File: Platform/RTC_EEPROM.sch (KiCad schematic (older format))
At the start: 21 parts, among them U4 DS3231M, U5 AT24CS32-SSHM, U6 MCP7940N-xMS, Y1 32KHz crystal

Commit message: updated.
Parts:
- BAT1: symbol Platform-rescue:BS-7-dk_Battery-Holders-Clips-Contacts -> Platform-rescue:BS-7-dk_Battery-Holders-Clips-Contacts-Platform-rescue
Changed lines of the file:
@@
 $EndComp
 $Comp
-L Platform-rescue:BS-7-dk_Battery-Holders-Clips-Contacts BAT1
+L Platform-rescue:BS-7-dk_Battery-Holders-Clips-Contacts-Platform-rescue BAT1
 U 1 1 5FB40A5C
 P 7500 1650

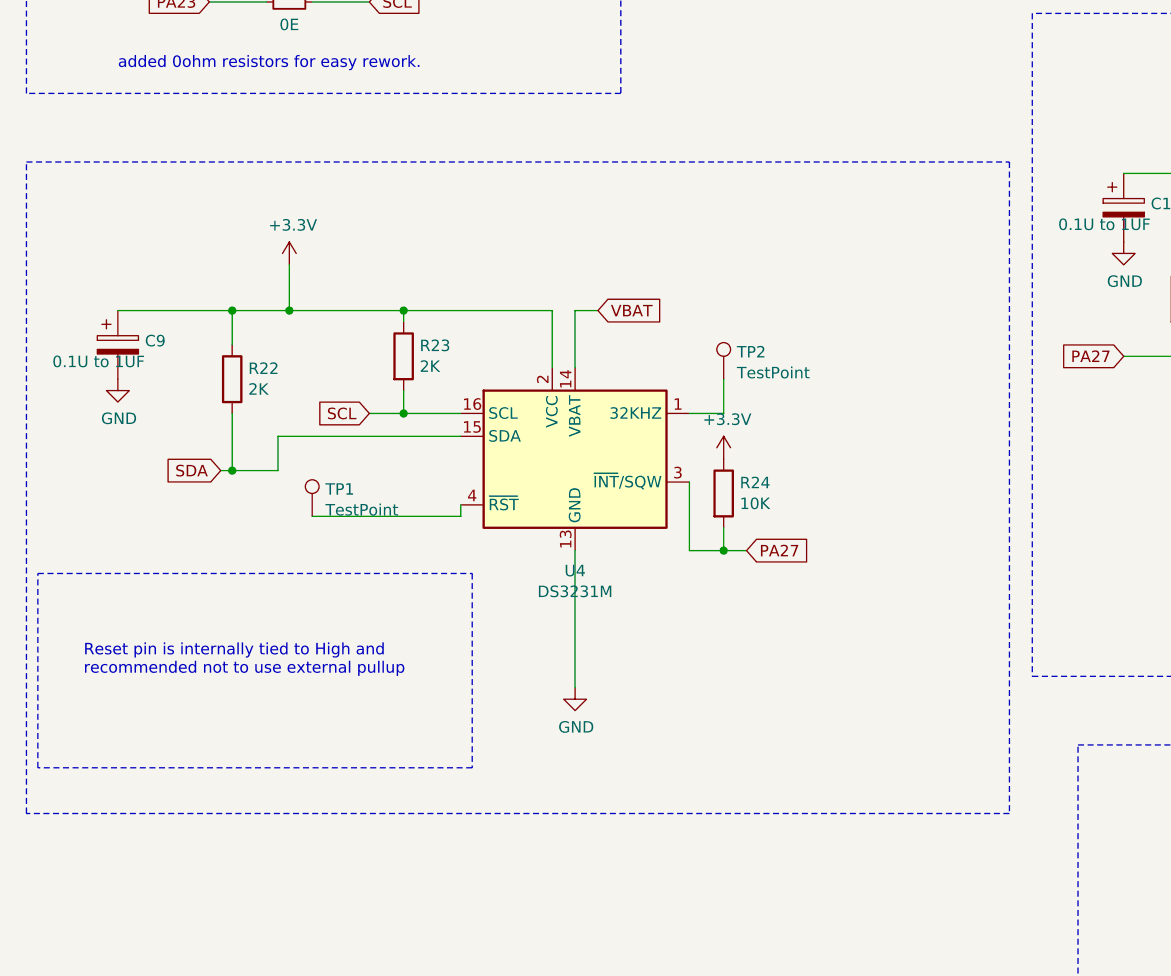
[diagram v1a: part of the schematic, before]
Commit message: Updated the schematic.
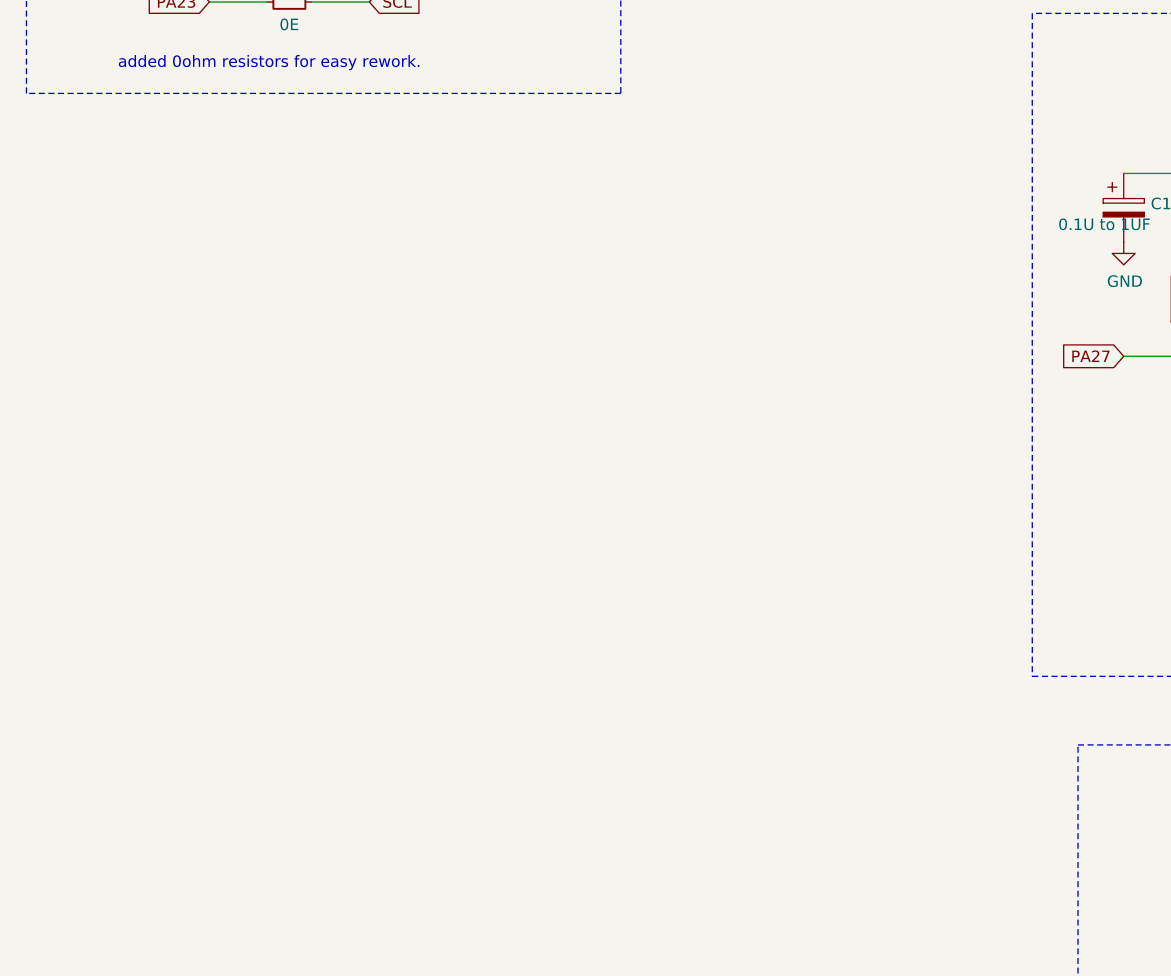
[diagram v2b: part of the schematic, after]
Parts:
- removed C9: 0.1U to 1UF, symbol Device:CP
- removed R22, R23: 2K, symbol Device:R
- removed R24: 10K, symbol Device:R
- removed TP1, TP2: TestPoint, symbol Connector:TestPoint
- removed U4: DS3231M, Package_SO:SOIC-16W_7.5x10.3mm_P1.27mm, symbol Timer_RTC:DS3231M
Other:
- note removed: "Reset pin is internally tied to High and \nrecommended not to use external pullup"
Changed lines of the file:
@@
 $EndDescr
-$Comp
-L Timer_RTC:DS3231M U4
-U 1 1 5FB09C8B
-P 2950 2900
-F 0 "U4" H 2950 2411 50  0000 C CNN
-F 1 "DS3231M" H 2950 2320 50  0000 C CNN
-F 2 "Package_SO:SOIC-16W_7.5x10.3mm_P1.27mm" H 2950 2300 50  0001 C CNN
-F 3 "http://datasheets.maximintegrated.com/en/ds/DS3231.pdf" H 3220 2950 50  0001 C CNN
-	1    2950 2900
-	1    0    0    -1
-$EndComp
-$Comp
-L power:+3.3V #PWR042
-U 1 1 5FB0AC4A
-P 1700 2050
-F 0 "#PWR042" H 1700 1900 50  0001 C CNN
-F 1 "+3.3V" H 1715 2223 50  0000 C CNN
-F 2 "" H 1700 2050 50  0001 C CNN
-F 3 "" H 1700 2050 50  0001 C CNN
-	1    1700 2050
-	1    0    0    -1
-$EndComp
-$Comp
-L power:GND #PWR043
-U 1 1 5FB0AFF3
-P 2950 3900
-F 0 "#PWR043" H 2950 3650 50  0001 C CNN
-F 1 "GND" H 2955 3727 50  0000 C CNN
-F 2 "" H 2950 3900 50  0001 C CNN
-F 3 "" H 2950 3900 50  0001 C CNN
-	1    2950 3900
-	1    0    0    -1
-$EndComp
-Wire Wire Line
-	1700 2050 1700 2250
-Wire Wire Line
-	1700 2250 2200 2250
-Wire Wire Line
-	2850 2250 2850 2500
-Text GLabel 2050 2700 0    50   Input ~ 0
-SCL
-Text GLabel 1400 2950 0    50   Input ~ 0
-SDA
-Wire Wire Line
-	1400 2950 1450 2950
-Wire Wire Line
-	1650 2950 1650 2800
-Wire Wire Line
-	1650 2800 2450 2800
-Wire Wire Line
-	2050 2700 2200 2700
-Wire Wire Line
-	2200 2300 2200 2250
-Connection ~ 2200 2250
-Wire Wire Line
-	2200 2250 2850 2250
-Wire Wire Line
-	2200 2600 2200 2700
-Connection ~ 2200 2700
-Wire Wire Line
-	2200 2700 2450 2700
-$Comp
-L Device:R R22
-U 1 1 5FB0C756
-P 1450 2550
-F 0 "R22" H 1520 2596 50  0000 L CNN
-F 1 "2K" H 1520 2505 50  0000 L CNN
-F 2 "" V 1380 2550 50  0001 C CNN
-F 3 "~" H 1450 2550 50  0001 C CNN
-	1    1450 2550
-	1    0    0    -1
-$EndComp
-Wire Wire Line
-	1450 2700 1450 2950
-Connection ~ 1450 2950
-Wire Wire Line
-	1450 2950 1650 2950
-Wire Wire Line
-	1450 2400 1450 2250
-Wire Wire Line
-	1450 2250 1700 2250
-Connection ~ 1700 2250
-$Comp
-L Device:CP C9
-U 1 1 5FB178E8
-P 950 2400
-F 0 "C9" H 1068 2446 50  0000 L TNN
-F 1 "0.1U to 1UF" H 1068 2355 50  0000 R TNN
-F 2 "" H 988 2250 50  0001 C CNN
-F 3 "~" H 950 2400 50  0001 C CNN
-	1    950  2400
-	1    0    0    -1
-$EndComp
-Wire Wire Line
-	950  2250 1450 2250
-Connection ~ 1450 2250
-$Comp
-L power:GND #PWR041
-U 1 1 5FB1839E
-P 950 2550
-F 0 "#PWR041" H 950 2300 50  0001 C CNN
-F 1 "GND" H 955 2377 50  0000 C CNN
-F 2 "" H 950 2550 50  0001 C CNN
-F 3 "" H 950 2550 50  0001 C CNN
-	1    950  2550
-	1    0    0    -1
-$EndComp
-$Comp
-L Device:R R23
-U 1 1 5FB0BB27
-P 2200 2450
-F 0 "R23" H 2270 2496 50  0000 L CNN
-F 1 "2K" H 2270 2405 50  0000 L CNN
-F 2 "" V 2130 2450 50  0001 C CNN
-F 3 "~" H 2200 2450 50  0001 C CNN
-	1    2200 2450
-	1    0    0    -1
-$EndComp
 $Comp
 L Timer:MCP7940N-xMS U6
@@
 	5350 2450 5600 2450
 Connection ~ 5600 2450
-Text GLabel 3700 3300 2    50   Input ~ 0
-PA27
-Wire Wire Line
-	2950 3300 2950 3900
-$Comp
-L Device:R R24
-U 1 1 5FB4ECAA
-P 3600 3050
-F 0 "R24" H 3670 3096 50  0000 L CNN
-F 1 "10K" H 3670 3005 50  0000 L CNN
-F 2 "" V 3530 3050 50  0001 C CNN
-F 3 "~" H 3600 3050 50  0001 C CNN
-	1    3600 3050
-	1    0    0    -1
-$EndComp
-$Comp
-L power:+3.3V #PWR044
-U 1 1 5FB4F46E
-P 3600 2900
-F 0 "#PWR044" H 3600 2750 50  0001 C CNN
-F 1 "+3.3V" H 3615 3073 50  0000 C CNN
-F 2 "" H 3600 2900 50  0001 C CNN
-F 3 "" H 3600 2900 50  0001 C CNN
-	1    3600 2900
-	1    0    0    -1
-$EndComp
-Wire Wire Line
-	3600 3200 3600 3300
-Wire Wire Line
-	3600 3300 3700 3300
-Wire Wire Line
-	3450 3000 3450 3300
-Wire Wire Line
-	3450 3300 3600 3300
-Connection ~ 3600 3300
 $Comp
 L Memory_EEPROM:AT24CS32-SSHM U5
@@
 	550  1300 550  600
 Wire Notes Line
-	4850 1600 4850 4450
-Wire Notes Line
-	4850 4450 550  4450
-Wire Notes Line
-	550  4450 550  1600
-Wire Notes Line
-	550  1600 4850 1600
-Wire Notes Line
 	4950 950  4950 3850
 Wire Notes Line
@@
 Wire Wire Line
 	7800 1850 7500 1850
-Wire Notes Line
-	2500 3400 2500 4250
-Wire Notes Line
-	2500 4250 600  4250
-Wire Notes Line
-	600  4250 600  3400
-Wire Notes Line
-	600  3400 2500 3400
-Text Notes 800  3850 0    50   ~ 0
-Reset pin is internally tied to High and \nrecommended not to use external pullup
-$Comp
-L Connector:TestPoint TP1
-U 1 1 5FB718D1
-P 1800 3150
-F 0 "TP1" H 1858 3268 50  0000 L CNN
-F 1 "TestPoint" H 1858 3177 50  0000 L CNN
-F 2 "" H 2000 3150 50  0001 C CNN
-F 3 "~" H 2000 3150 50  0001 C CNN
-	1    1800 3150
-	1    0    0    -1
-$EndComp
-Wire Wire Line
-	1800 3150 2450 3150
-Wire Wire Line
-	2450 3150 2450 3100
-$Comp
-L Connector:TestPoint TP2
-U 1 1 5FB7652B
-P 3600 2550
-F 0 "TP2" H 3658 2668 50  0000 L CNN
-F 1 "TestPoint" H 3658 2577 50  0000 L CNN
-F 2 "" H 3800 2550 50  0001 C CNN
-F 3 "~" H 3800 2550 50  0001 C CNN
-	1    3600 2550
-	1    0    0    -1
-$EndComp
-Wire Wire Line
-	3600 2550 3600 2700
-Wire Wire Line
-	3600 2700 3450 2700
 $Comp
 L Device:R_Small R30
@@
 	7500 1300 7500 1450
 Connection ~ 7500 1450
-Text GLabel 3050 2250 2    50   Input ~ 0
-VBAT
-Wire Wire Line
-	3050 2250 2950 2250
-Wire Wire Line
-	2950 2250 2950 2500
 $Comp
 L Device:C_Small C11
